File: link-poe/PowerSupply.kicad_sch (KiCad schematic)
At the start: 8 parts, among them U501 TPSM33625

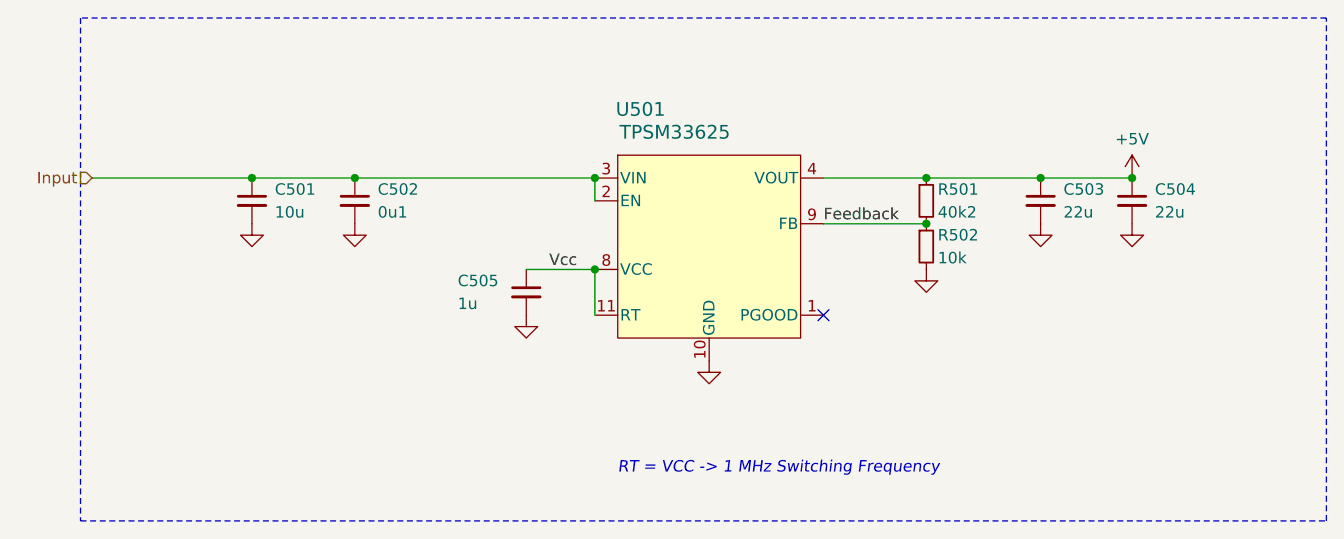
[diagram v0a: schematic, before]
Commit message: Update parts
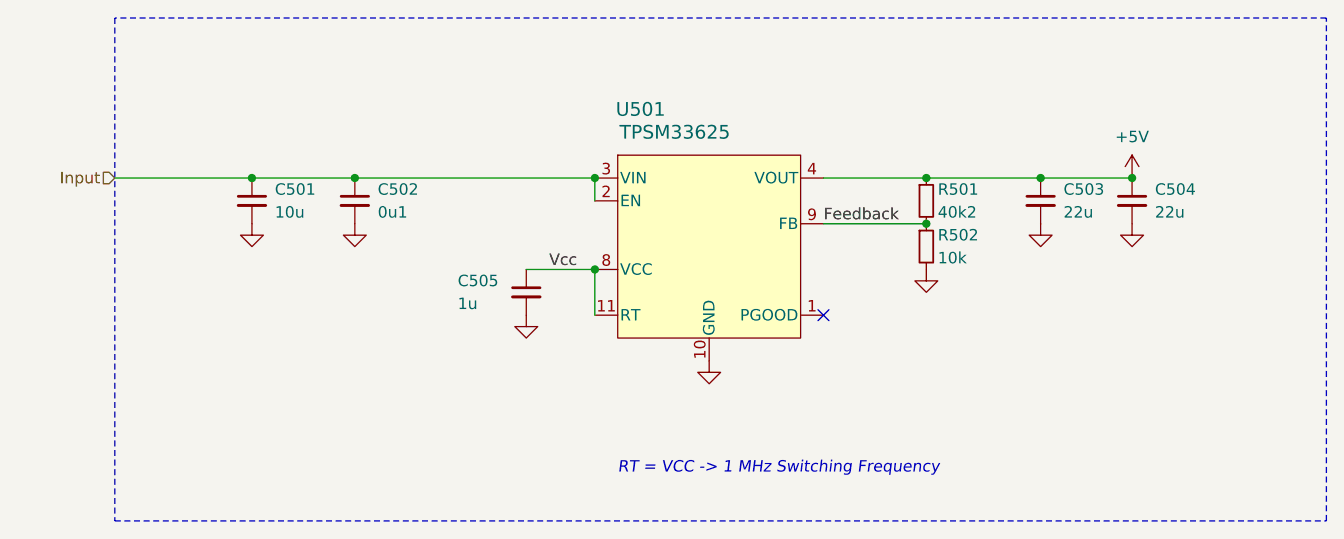
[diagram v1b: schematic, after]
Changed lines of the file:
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@@
 	(wire
 		(pts
-			(xy 80.01 95.25) (xy 97.79 95.25)
+			(xy 82.55 95.25) (xy 97.79 95.25)
 		)
 		(stroke
@@
 	(polyline
 		(pts
-			(xy 78.74 77.47) (xy 78.74 133.35)
+			(xy 82.55 77.47) (xy 82.55 133.35)
 		)
 		(stroke
@@
 	(polyline
 		(pts
-			(xy 78.74 133.35) (xy 217.17 133.35)
+			(xy 82.55 133.35) (xy 217.17 133.35)
 		)
 		(stroke
@@
 	(polyline
 		(pts
-			(xy 217.17 77.47) (xy 78.74 77.47)
+			(xy 217.17 77.47) (xy 82.55 77.47)
 		)
 		(stroke
@@
 	(hierarchical_label "Input"
 		(shape input)
-		(at 80.01 95.25 180)
+		(at 82.55 95.25 180)
 		(effects
 			(font
@@
 		)
 		(property "Value" "+5V"
-			(at 195.58 90.932 0)
-			(effects
-				(font
+			(at 195.58 90.678 0)
+			(effects
+				(font

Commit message: Refresh
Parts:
- C501: Manufacturer (none) -> TDK; Product (none) -> CNA6P1X7R1H106K250AE; Rating 50V -> (none); Voltage (none) -> 50V
- C502: Manufacturer (none) -> TDK; Product (none) -> CGA3E2X7R1H104M080AA
- C503, C504: Manufacturer (none) -> TDK; Product (none) -> CGA6P3X7R1E226M250AE; Rating 25V -> (none); Voltage (none) -> 25V
- C505: Manufacturer (none) -> YAGEO; Mouser 810-CGA3E2X7R1H104MA -> 603-CC603KRX7R9BB105; Product (none) -> CC0603KRX7R9BB105
- R501: Manufacturer (none) -> Vishay; Product (none) -> RCS060340K2FKEA; Rating (none) -> 500mW
- R502: Manufacturer (none) -> Vishay; Product (none) -> CRCW060310K0FKEAC; Rating (none) -> 100mW
- U501: Manufacturer (none) -> Texas Instruments; Product (none) -> TPSM33625RDNR
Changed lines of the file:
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@@
+			)
+		)
+		(property "Manufacturer" "Texas Instruments"
+			(at 148.59 146.05 0)
+			(effects
+				(font
+					(size 1.27 1.27)
+				)
+				(hide yes)
+			)
+		)
+		(property "Product" "TPSM33625RDNR"
+			(at 148.59 148.59 0)
+			(effects
+				(font
+					(size 1.27 1.27)
+				)
+				(hide yes)
 			)
 		)
@@
 			)
 		)
+		(property "Manufacturer" "TDK"
+			(at 109.22 113.03 0)
+			(effects
+				(font
+					(size 1.27 1.27)
+				)
+				(hide yes)
+			)
+		)
+		(property "Product" "CGA3E2X7R1H104M080AA"
+			(at 109.22 115.57 0)
+			(effects
+				(font
+					(size 1.27 1.27)
+				)
+				(hide yes)
+			)
+		)
 		(pin "1"
 		)
@@
 			)
 		)
-		(property "Rating" "25V"
-			(at 195.58 117.094 0)
+		(property "Voltage" "25V"
+			(at 195.58 118.11 0)
+			(effects
+				(font
+					(size 1.27 1.27)
+				)
+				(hide yes)
+			)
+		)
+		(property "Product" "CGA6P3X7R1E226M250AE"
+			(at 195.58 115.57 0)
+			(effects
+				(font
+					(size 1.27 1.27)
+				)
+				(hide yes)
+			)
+		)
+		(property "Manufacturer" "TDK"
+			(at 195.58 113.03 0)
 			(effects
 				(font
@@
 			)
 		)
+		(property "Rating" "500mW"
+			(at 172.72 118.11 0)
+			(effects
+				(font
+					(size 1.27 1.27)
+				)
+				(hide yes)
+			)
+		)
+		(property "Manufacturer" "Vishay"
+			(at 172.72 113.03 0)
+			(effects
+				(font
+					(size 1.27 1.27)
+				)
+				(hide yes)
+			)
+		)
+		(property "Product" "RCS060340K2FKEA"
+			(at 172.72 115.57 0)
+			(effects
+				(font
+					(size 1.27 1.27)
+				)
+				(hide yes)
+			)
+		)
 		(pin "1"
 		)
@@
 			)
 		)
-		(property "Mouser" "810-CGA3E2X7R1H104MA"
+		(property "Mouser" "603-CC603KRX7R9BB105"
 			(at 128.27 125.222 0)
+			(effects
+				(font
+					(size 1.27 1.27)
+				)
+				(hide yes)
+			)
+		)
+		(property "Product" "CC0603KRX7R9BB105"
+			(at 128.27 125.73 0)
+			(effects
+				(font
+					(size 1.27 1.27)
+				)
+				(hide yes)
+			)
+		)
+		(property "Manufacturer" "YAGEO"
+			(at 128.27 123.19 0)
 			(effects
 				(font
@@
 			)
 		)
-		(property "Rating" "25V"
-			(at 189.738 101.6 0)
+		(property "Voltage" "25V"
+			(at 185.42 118.11 0)
+			(effects
+				(font
+					(size 1.27 1.27)
+				)
+				(hide yes)
+			)
+		)
+		(property "Product" "CGA6P3X7R1E226M250AE"
+			(at 185.42 115.57 0)
+			(effects
+				(font
+					(size 1.27 1.27)
+				)
+				(hide yes)
+			)
+		)
+		(property "Manufacturer" "TDK"
+			(at 185.42 113.03 0)
 			(effects
 				(font
@@
 			)
 		)
+		(property "Product" "CRCW060310K0FKEAC"
+			(at 172.72 120.65 0)
+			(effects
+				(font
+					(size 1.27 1.27)
+				)
+				(hide yes)
+			)
+		)
+		(property "Manufacturer" "Vishay"
+			(at 172.72 118.11 0)
+			(effects
+				(font
+					(size 1.27 1.27)
+				)
+				(hide yes)
+			)
+		)
+		(property "Rating" "100mW"
+			(at 172.72 123.19 0)
+			(effects
+				(font
+					(size 1.27 1.27)
+				)
+				(hide yes)
+			)
+		)
 		(pin "1"
 		)
@@
 			)
 		)
-		(property "Rating" "50V"
-			(at 102.108 102.108 0)
-			(effects
-				(font
+		(property "Voltage" "50V"
+			(at 97.79 118.11 0)
+			(effects
+				(font
+					(size 1.27 1.27)
+				)
+				(hide yes)
+			)
+		)
+		(property "Product" "CNA6P1X7R1H106K250AE"
+			(at 97.79 115.57 0)
+			(effects
+				(font
+					(size 1.27 1.27)
+				)
+				(hide yes)
+			)
+		)
+		(property "Manufacturer" "TDK"
+			(at 97.79 113.03 0)
+			(effects
+				(font

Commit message: Fix WAGOs
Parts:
- C505: Rating (none) -> 50V
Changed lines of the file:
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@@
+			)
+		)
+		(property "Rating" "50V"
+			(at 128.27 130.81 0)
+			(effects
+				(font
+					(size 1.27 1.27)
+				)
+				(hide yes)
 			)
 		)

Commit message: Refresh
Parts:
- C501: Rating (none) -> 50V; Voltage 50V -> (none)
- C502: Rating (none) -> 50V
- C503, C504: Rating (none) -> 25V; Voltage 25V -> (none)
- C505: Manufacturer YAGEO -> TDK; Mouser 603-CC603KRX7R9BB105 -> 810-CGA3E3X7R1H105K0; Product CC0603KRX7R9BB105 -> CGA3E3X7R1H105K080AB
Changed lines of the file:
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@@
+			)
+		)
+		(property "Rating" "50V"
+			(at 109.22 120.65 0)
+			(effects
+				(font
+					(size 1.27 1.27)
+				)
+				(hide yes)
 			)
 		)
@@
 			)
 		)
-		(property "Voltage" "25V"
-			(at 195.58 118.11 0)
-			(effects
-				(font
-					(size 1.27 1.27)
-				)
-				(hide yes)
-			)
-		)
 		(property "Product" "CGA6P3X7R1E226M250AE"
 			(at 195.58 115.57 0)
@@
 			)
 		)
+		(property "Rating" "25V"
+			(at 195.58 118.11 0)
+			(effects
+				(font
+					(size 1.27 1.27)
+				)
+				(hide yes)
+			)
+		)
 		(pin "1"
 		)
@@
 			)
 		)
-		(property "Mouser" "603-CC603KRX7R9BB105"
+		(property "Mouser" "810-CGA3E3X7R1H105K0"
 			(at 128.27 125.222 0)
 			(effects
@@
 			)
 		)
-		(property "Product" "CC0603KRX7R9BB105"
+		(property "Product" "CGA3E3X7R1H105K080AB"
 			(at 128.27 125.73 0)
 			(effects
@@
 			)
 		)
-		(property "Manufacturer" "YAGEO"
+		(property "Manufacturer" "TDK"
 			(at 128.27 123.19 0)
 			(effects
@@
 			)
 		)
-		(property "Voltage" "25V"
-			(at 185.42 118.11 0)
-			(effects
-				(font
-					(size 1.27 1.27)
-				)
-				(hide yes)
-			)
-		)
 		(property "Product" "CGA6P3X7R1E226M250AE"
 			(at 185.42 115.57 0)
@@
 			)
 		)
+		(property "Rating" "25V"
+			(at 185.42 118.11 0)
+			(effects
+				(font
+					(size 1.27 1.27)
+				)
+				(hide yes)
+			)
+		)
 		(pin "1"
 		)
@@
 			)
 		)
-		(property "Voltage" "50V"
-			(at 97.79 118.11 0)
-			(effects
-				(font
-					(size 1.27 1.27)
-				)
-				(hide yes)
-			)
-		)
 		(property "Product" "CNA6P1X7R1H106K250AE"
 			(at 97.79 115.57 0)
@@
 			(effects
 				(font
+					(size 1.27 1.27)
+				)
+				(hide yes)
+			)
+		)
+		(property "Rating" "50V"
+			(at 97.79 118.11 0)
+			(effects
+				(font
